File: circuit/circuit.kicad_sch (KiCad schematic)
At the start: 15 parts

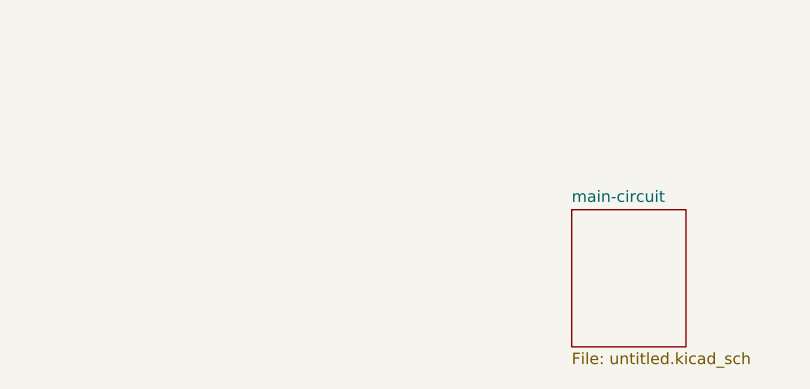
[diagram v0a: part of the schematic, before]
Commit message: WIP
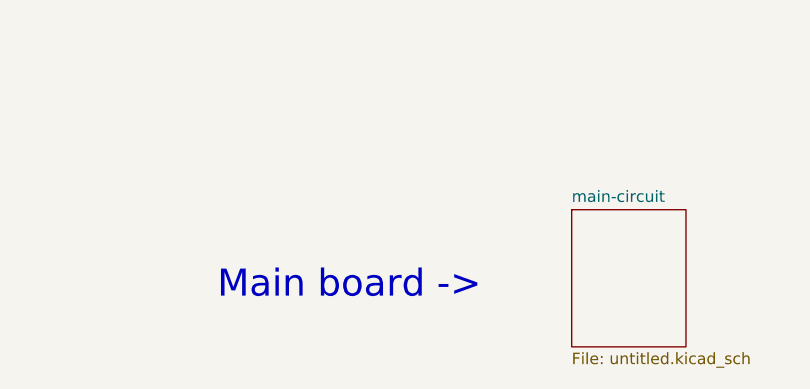
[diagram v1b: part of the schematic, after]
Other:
- note added: "Main board ->"
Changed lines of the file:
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@@
     (effects (font (size 3 3) (thickness 0.6) bold) (justify left bottom))
+  )
+  (text "Main board ->" (at 111.76 186.69 0)
+    (effects (font (size 3 3)) (justify left bottom))
   )
   (text "Wires:\nRED    -- VCC\nBLACK  -- GND\nYELLOW -- DATA\nORANGE -- ADDR\nGREEN  -- SPI\nPURPLE -- Z80 BUS\nBROWN  -- SERIAL\nBLUE   -- OTHER"
@@
       (reference "#PWR?") (unit 1) (value "+5V") (footprint "")
     )
+    (path "/e9d70090-90fc-4e9b-9b66-2c4a5e914581/8667c096-1105-4282-abf5-b5f5fd5d95a1"
+      (reference "#PWR?") (unit 1) (value "+3V3") (footprint "")
+    )
     (path "/e9d70090-90fc-4e9b-9b66-2c4a5e914581/883247fb-bfb5-42ae-8659-a110c018d3aa"
       (reference "#PWR?") (unit 1) (value "+5V") (footprint "")
@@
       (reference "#PWR?") (unit 1) (value "+5V") (footprint "")
     )
+    (path "/e9d70090-90fc-4e9b-9b66-2c4a5e914581/ea43ba8b-e61d-4888-aa80-16b0815f20c3"
+      (reference "#PWR?") (unit 1) (value "+5V") (footprint "")
+    )
     (path "/e9d70090-90fc-4e9b-9b66-2c4a5e914581/eac37082-9088-47ba-ac7c-ed45350bdf21"
       (reference "#PWR?") (unit 1) (value "+5V") (footprint "")
@@
       (reference "U?") (unit 1) (value "ATmega2560-16A") (footprint "Package_QFP:TQFP-100_14x14mm_P0.5mm")
     )
+    (path "/e9d70090-90fc-4e9b-9b66-2c4a5e914581/e6bc2f02-5b3d-4456-a918-ddd7fc18f8e5"
+      (reference "U?") (unit 1) (value "Level shifter") (footprint "Package_SO:TSSOP-14_4.4x5mm_P0.65mm")
+    )
     (path "/e9d70090-90fc-4e9b-9b66-2c4a5e914581/b78b446a-b4b4-477c-99a7-ae017f47fd2e"
